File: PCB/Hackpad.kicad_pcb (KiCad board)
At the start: 2 copper layers, 83.3 x 66.7 mm, 7 parts, among them SW1 SW_Push, SW2 SW_Push, SW3 SW_Push, SW4 SW_Push, U1 XIAO-RP2040-DIP

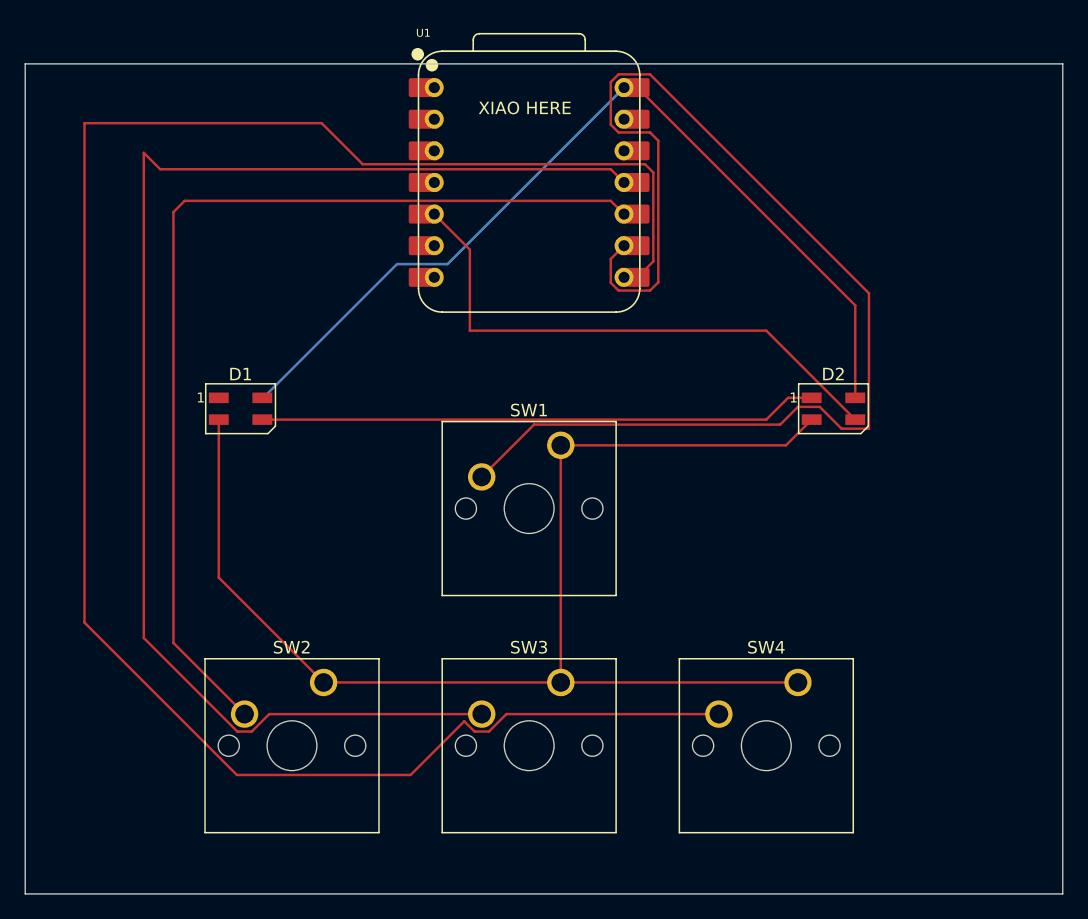
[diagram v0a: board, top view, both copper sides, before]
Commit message: wiring better
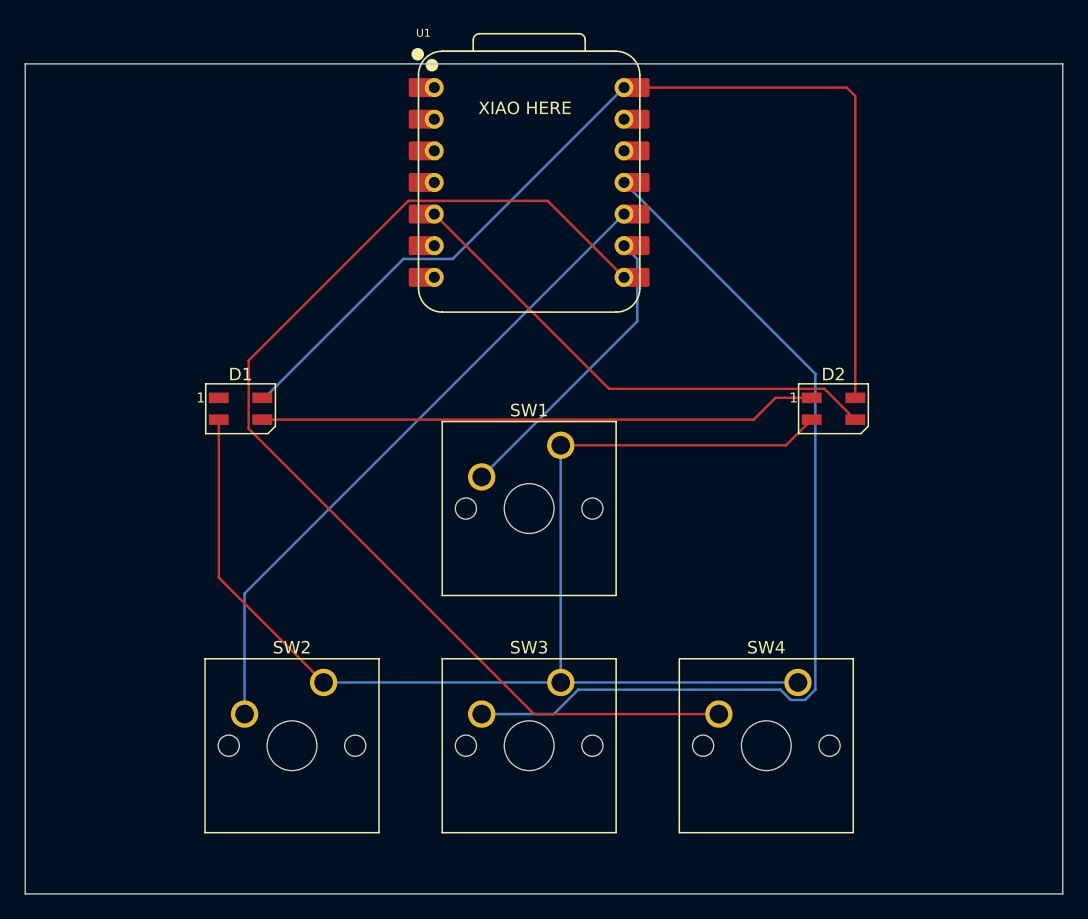
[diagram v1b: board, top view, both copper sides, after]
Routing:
- net Net-(U1-GPIO2/SCK): track 100.2 -> 24.2 mm
- net Net-(U1-GPIO1/RX): track 156.2 -> 91.8 mm
- net Net-(U1-GPIO3/MOSI): track 109.4 -> 75.4 mm
- net Net-(U1-GPIO4/MISO): track 79.7 -> 52.8 mm
- net +5V: track 72.6 -> 82.5 mm
- net Net-(D2-DIN): track 44.5 -> 40.7 mm
